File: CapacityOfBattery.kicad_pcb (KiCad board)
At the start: 2 copper layers, 28 parts, among them J1 BATTERY, J2 DUT, Q1 IRLML6401TRPBF, Q2 IRLML6401TRPBF, Q3 IRLML6401TRPBF, Q4 IRLML6401TRPBF, Q5 SI2302, SW1 SW_Push

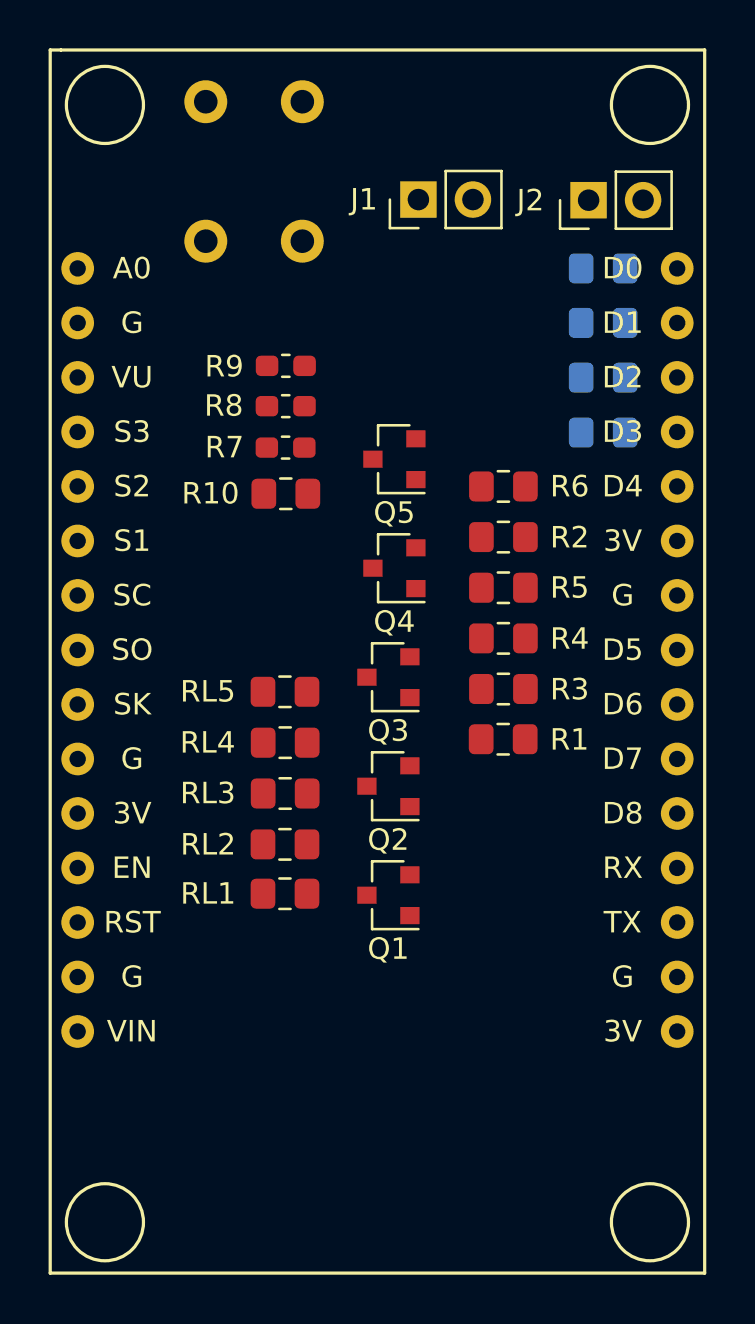
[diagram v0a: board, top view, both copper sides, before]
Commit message: pcb updated
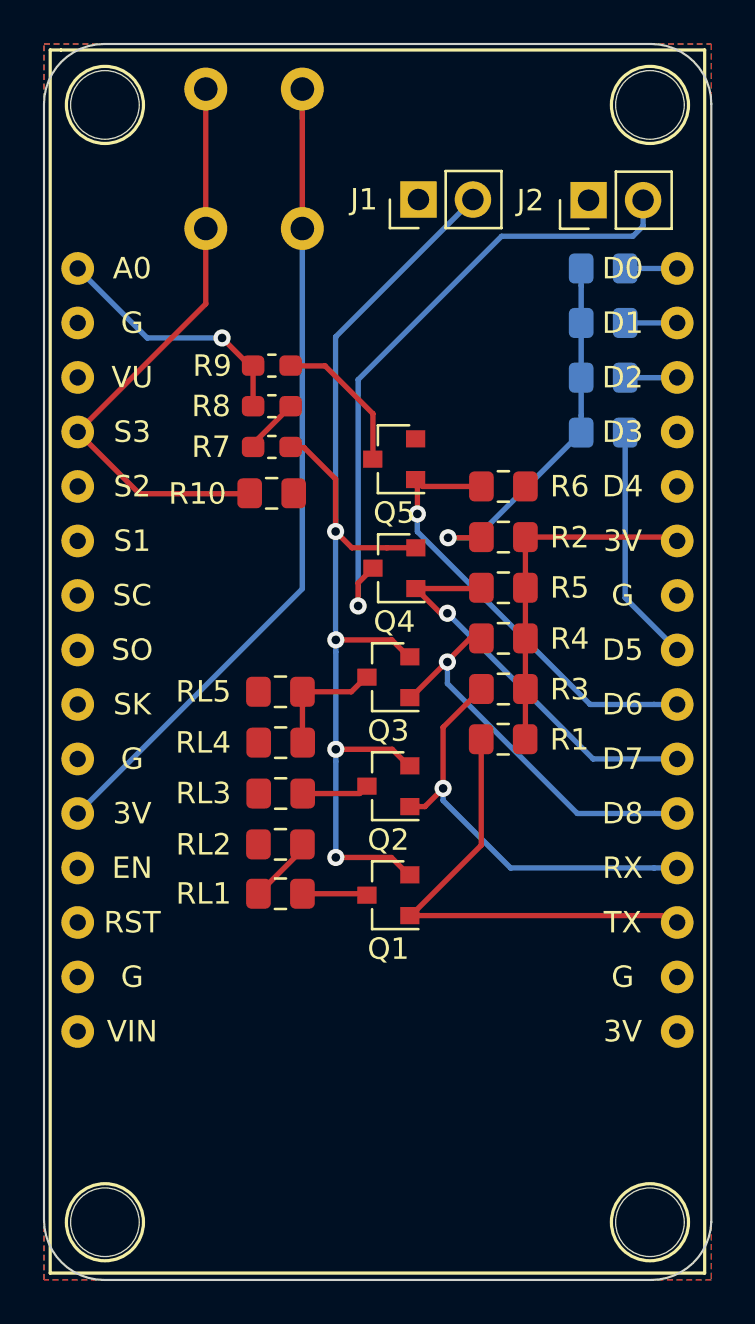
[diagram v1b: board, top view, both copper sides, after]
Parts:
- added ?: MountingHole_3.2mm_M3_ISO7380, MountingHole:MountingHole_3.2mm_M3_ISO7380, F.Cu at (41.5, 67.3)
- added ?: MountingHole_3.2mm_M3_ISO7380, MountingHole:MountingHole_3.2mm_M3_ISO7380, F.Cu at (16.1, 67.3)
- added ?: MountingHole_3.2mm_M3_ISO7380, MountingHole:MountingHole_3.2mm_M3_ISO7380, F.Cu at (16.1, 15.2)
- added ?: MountingHole_3.2mm_M3_ISO7380, MountingHole:MountingHole_3.2mm_M3_ISO7380, F.Cu at (41.5, 15.2)
- Q5: value SI2302 -> SOT-23
- R10: value 1k -> R_0805_2012Metric_Pad1.15x1.40mm_HandSolder
- R7, R8, R9: value 30k -> R_0603_1608Metric_Pad1.05x0.95mm_HandSolder
- moved R10 0.66 mm to (23.9, 33.3)
- moved R9 0.65 mm to (23.9, 27.4)
- moved R8 0.65 mm to (23.9, 29.3)
- moved R7 0.64 mm to (23.9, 31.2)
- moved SW1 0.59 mm to (25.3, 21.0)
- moved RL1 0.21 mm to (24.3, 52.0)
- moved RL2 0.21 mm to (24.3, 49.7)
- moved RL3 0.21 mm to (24.3, 47.3)
- moved RL4 0.21 mm to (24.3, 45.0)
- moved RL5 0.21 mm to (24.3, 42.6)
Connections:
- R8 pad 1: Net-(R7-Pad2) -> /Vin
- R8 pad 2: /Vin -> Net-(R7-Pad2)
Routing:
- net /Vcc: track 0.00 -> 56.1 mm
- net /Vbat: track 0.00 -> 53.8 mm, vias 0 -> 4
- net /dut: track 0.00 -> 30.0 mm, vias 0 -> 1
- net /SW: track 0.00 -> 27.7 mm
- net /Ctrl1: track 0.00 -> 22.2 mm
- net /En_VD: track 0.00 -> 21.1 mm, vias 0 -> 1
- net /Ctrl2: track 0.00 -> 20.0 mm, vias 0 -> 1
- net /Ctrl3: track 0.00 -> 18.7 mm, vias 0 -> 1
- net /Ctrl4: track 0.00 -> 18.6 mm, vias 0 -> 1
- net Net-(D1-Pad2): track 0.00 -> 17.5 mm, vias 0 -> 1
- net /Vin: track 0.00 -> 11.9 mm, vias 0 -> 1
- net /LED4: track 0.00 -> 11.1 mm
- net Net-(Q5-Pad3): track 0.00 -> 6.87 mm
- net Net-(Q3-Pad3): track 0.00 -> 5.66 mm
- net Net-(RL1-Pad2): track 0.00 -> 3.15 mm
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- added copper zone on B.Cu, net GND
- added copper zone on F.Cu, net GND
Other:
- board outline added: 31.1 x 57.6 mm
